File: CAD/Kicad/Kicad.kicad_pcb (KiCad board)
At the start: 6 copper layers, 69.5 x 63 mm, 38 parts, among them J1 USB_C_Receptacle_USB2.0_14P, J2 USB_C_Receptacle_USB2.0_14P, J3 Conn_01x20_Pin, J4 Conn_01x20_Pin, J6 RJ45, Q1 2N3904, Q2 2N3904, SW1 SW_Push, SW2 SW_Push, U1 ESP32-S3-WROOM-2, U3 AMS1117-3.3, U7 BME680, U8 MPU-9250, U9 FT231XQ

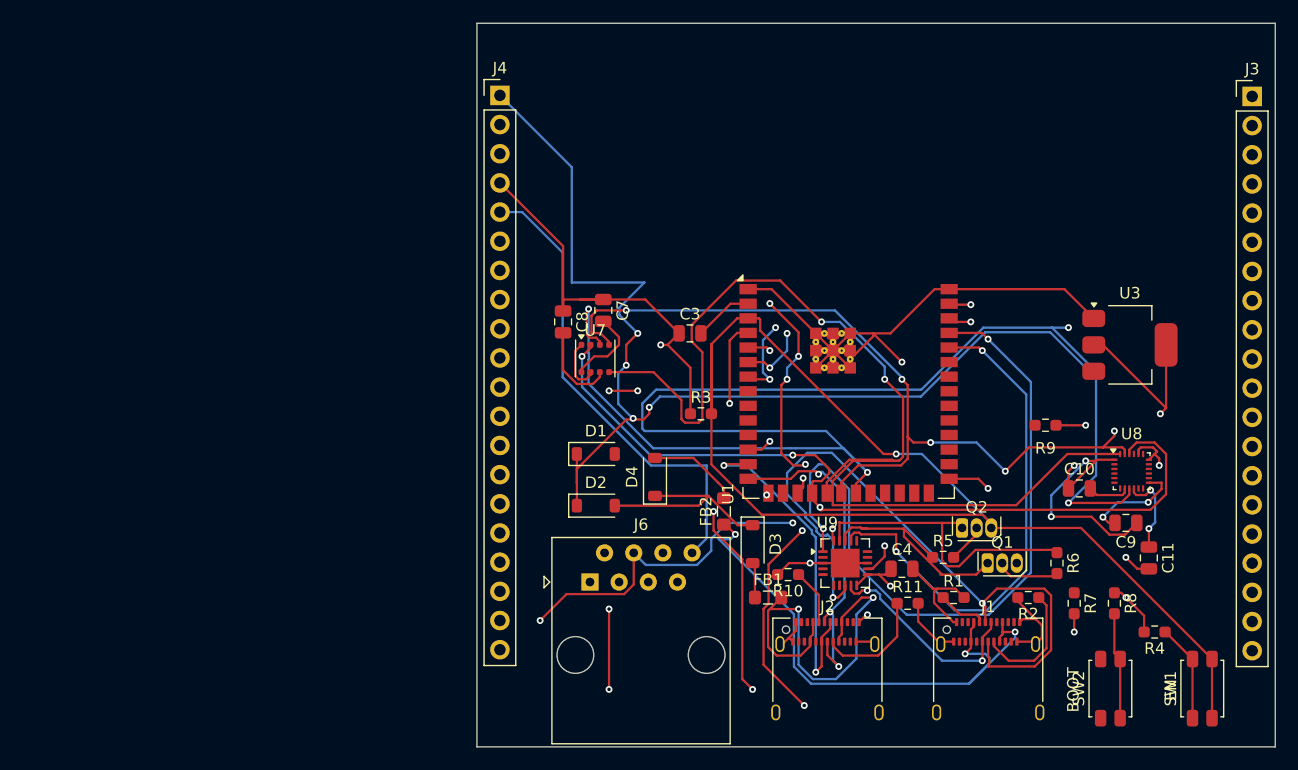
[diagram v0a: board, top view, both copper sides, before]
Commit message: Finalized PCB (Yes!)
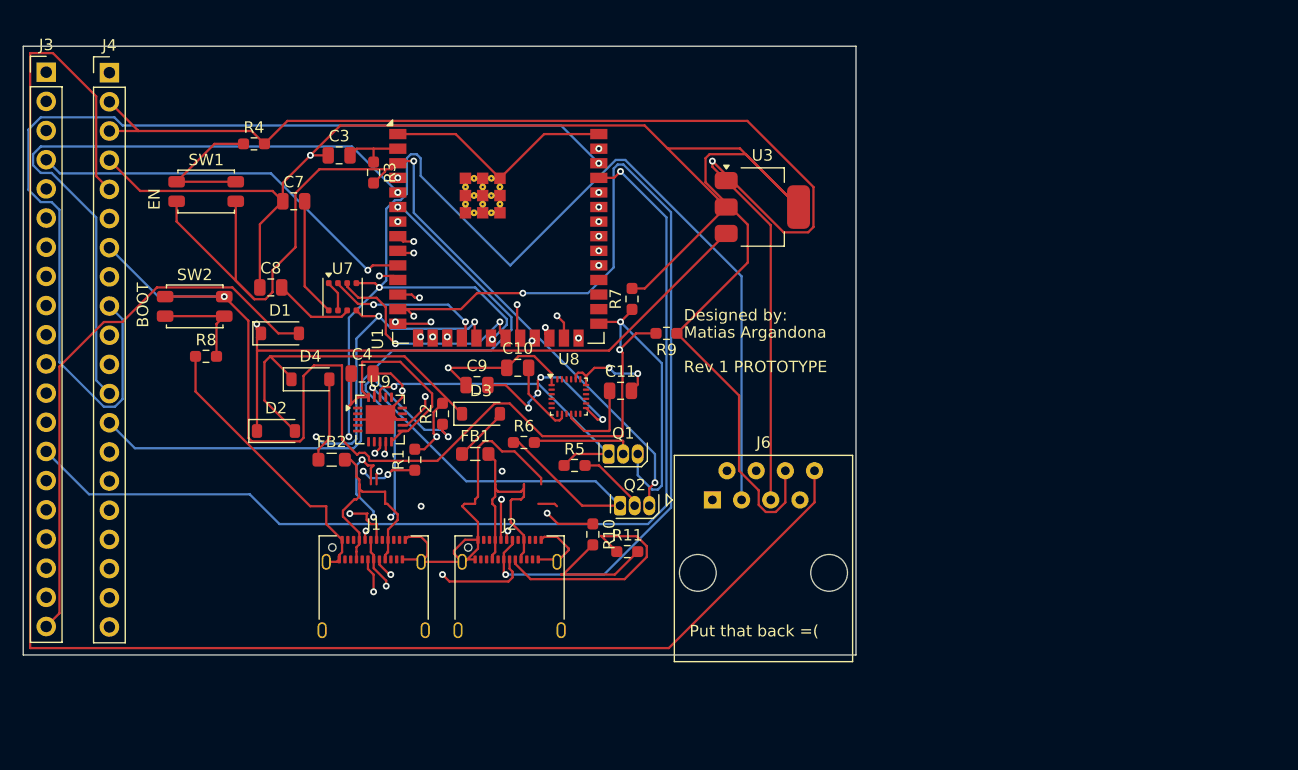
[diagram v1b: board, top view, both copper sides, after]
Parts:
- moved J3 105.0 mm to (125.0, 34.8)
- moved SW1 96.9 mm to (138.9, 45.1), turned to 0 degrees
- moved R4 89.2 mm to (143.1, 41.0), turned to 0 degrees
- moved SW2 86.4 mm to (137.9, 55.1), turned to 0 degrees
- moved R8 82.0 mm to (138.9, 59.5), turned to 0 degrees
- moved C9 57.8 mm to (162.5, 62.0), turned to 0 degrees
- moved J1 54.0 mm to (153.5, 80.5)
- moved R2 53.5 mm to (159.5, 64.5), turned to 90 degrees
- moved C10 50.0 mm to (166.1, 60.5)
- moved C4 50.0 mm to (152.5, 61.0)
- moved U8 49.4 mm to (170.5, 63.0)
- moved R1 48.4 mm to (157.1, 68.5), turned to 90 degrees
- moved C11 48.2 mm to (175.0, 62.5), turned to 0 degrees
- moved R6 47.6 mm to (166.6, 67.0), turned to 0 degrees
- moved R7 46.7 mm to (176.0, 54.5), turned to 90 degrees
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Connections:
- U9 pad 14: /CBUS1 -> unconnected-(U9-CBUS1-Pad14)
- U9 pad 15: /CBUS0 -> unconnected-(U9-CBUS0-Pad15)
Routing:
- net /VCC0: track 86.9 -> 200.9 mm, vias 8 -> 3
- net /RJ43_P8: track 41.6 -> 144.0 mm
- net /GND: track 216.8 -> 316.6 mm
- net /IO9: track 136.3 -> 36.8 mm, vias 5 -> 1
- net /NATIVE_D-: track 29.5 -> 128.5 mm, vias 2 -> 3
- net /IO3: track 113.8 -> 27.2 mm
- net /IO7: track 116.4 -> 33.4 mm, vias 2 -> 1
- net /MISO_BUS_A: track 213.9 -> 134.0 mm, vias 4 -> 2
- net /NATIVE_D+: track 29.2 -> 102.5 mm, vias 3 -> 4
- net /IO48: track 0.00 -> 73.0 mm, vias 0 -> 1
- net /IO47: track 0.00 -> 69.5 mm, vias 0 -> 1
- net /IO42: track 0.00 -> 64.9 mm, vias 0 -> 1
- net /IO41: track 0.00 -> 62.7 mm, vias 0 -> 1
- net /IO40: track 0.00 -> 61.3 mm, vias 0 -> 1
- net /IO39: track 0.00 -> 60.3 mm, vias 0 -> 1
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- removed copper zone on In2.Cu, net /VCC0
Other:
- board size 69.5 x 63 mm -> 72.5 x 53 mm
- board text added: "Designed by:"
- board text added: "Matias Argandona"
- board text added: "Put that back =("
- board text added: "Rev 1 PROTOTYPE"
